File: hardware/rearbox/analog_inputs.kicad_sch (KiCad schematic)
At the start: 4 parts

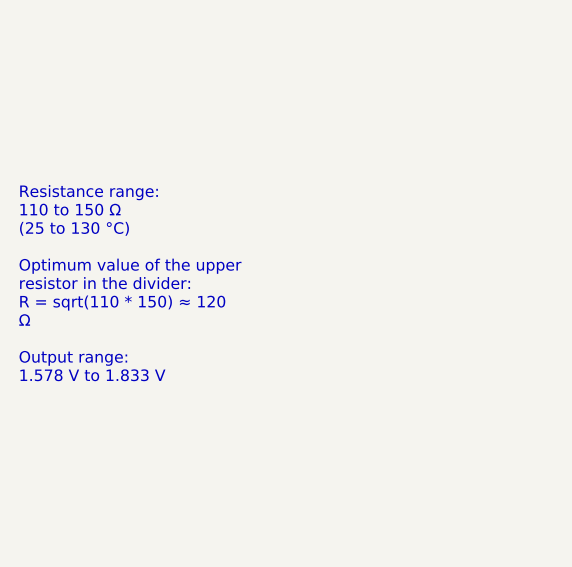
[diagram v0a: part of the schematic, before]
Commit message: Changed power section
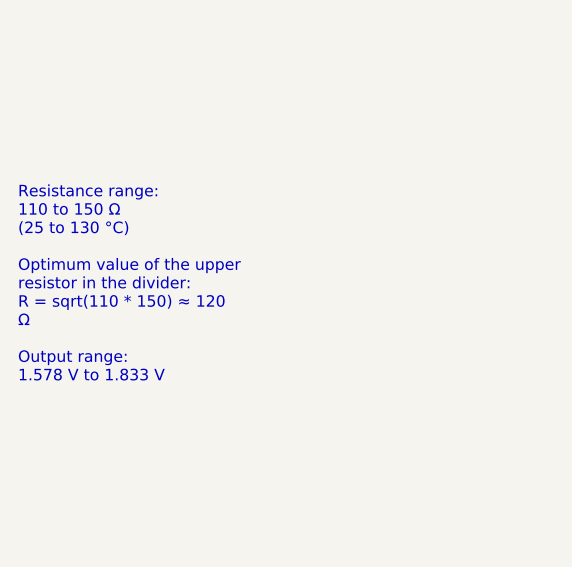
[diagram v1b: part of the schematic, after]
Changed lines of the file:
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@@
 (kicad_sch
-	(version 20231120)
+	(version 20250114)
 	(generator "eeschema")
-	(generator_version "8.0")
+	(generator_version "9.0")
 	(paper "A4")
 	(title_block
@@
 		(company "Author: I. Kajdan")
 		(comment 1 "Reviewer:")
+	)
+	(text "PT100"
+		(exclude_from_sim no)
+		(at 170.18 73.66 0)
+		(effects
+			(font
+				(size 1.27 1.27)
+			)
+			(justify right bottom)
+		)
+	)
+	(text "PT100"
+		(exclude_from_sim no)
+		(at 170.18 127 0)
+		(effects
+			(font
+				(size 1.27 1.27)
+			)
+			(justify right bottom)
+		)
+	)
+	(text "G = 2\nR_{F} = 4k7\nR_{G} = 4k7"
+		(exclude_from_sim no)
+		(at 204.47 87.63 0)
+		(effects
+			(font
+				(size 1.27 1.27)
+			)
+			(justify left bottom)
+		)
+	)
+	(text "G = 2\nR_{F} = 4k7\nR_{G} = 4k7"
+		(exclude_from_sim no)
+		(at 204.47 140.97 0)
+		(effects
+			(font
+				(size 1.27 1.27)
+			)
+			(justify left bottom)
+		)
+	)
+	(text_box "Resistance range:\n110 to 150 Ω\n(25 to 130 °C)\n\nOptimum value of the upper resistor in the divider:\nR = sqrt(110 * 150) ≈ 120 Ω\n\nOutput range:\n1.578 V to 1.833 V"
+		(exclude_from_sim no)
+		(at 48.26 99.06 0)
+		(size 31.75 22.86)
+		(margins 0.9524 0.9524 0.9524 0.9524)
+		(stroke
+			(width -0.0001)
+			(type default)
+		)
+		(fill
+			(type none)
+		)
+		(effects
+			(font
+				(size 1.27 1.27)
+			)
+			(justify left top)
+		)
 	)
 	(junction
@@
 			"FqxEIhEKhXw+Hz6Lx+MT2VgOh8PhcDiczwIIbPf5fJFIRK1WC4KQTCZVsF0xxpRKZTAYDAaDE91O"
 			"DofD4XA4nM8earWaSVFZPNCKw+FwOBwOZ4zhAovD4XA4HA5njOECi8PhcDgcDmeM+X+zbrmZJZpn"
-			"oAAAAABJRU5ErkJggg=="
-		)
-	)
-	(text_box "Resistance range:\n110 to 150 Ω\n(25 to 130 °C)\n\nOptimum value of the upper resistor in the divider:\nR = sqrt(110 * 150) ≈ 120 Ω\n\nOutput range:\n1.578 V to 1.833 V"
-		(exclude_from_sim no)
-		(at 48.26 99.06 0)
-		(size 31.75 22.86)
-		(stroke
-			(width -0.0001)
-			(type default)
-		)
-		(fill
-			(type none)
-		)
+			"oAAAAABJRU5ErkJgggB5AGsAZABHAEgAagBFAHQAWABzAC8AMQBRADYAUQBYAHUAQwBTAEoAVQB2"
+			"ADIANwBkAHQASABLAFUAMABrAEUAbgBQAG4AegBwADAAegBaAHcANgBsAEYAQwAxAEgATwBwADMA"
+			"RwBtAFkATwBtAEkAaAA2AFAAKwA2AHUANQBZAEIATQBTAGkAVQBSAFgAVgB4AGMAVwB6AHMARgB6"
+			"AHgAZgBpAGsAMABkAEoAYgBsAGkAVwBQAHYAOABHAEEASAB0AEQARAB2AGoAVgBOAEUAegAwAC8A"
+			"bgBQAGwAWQBTAGsAUAA0AGEAbAA3AEwASAB3AFoASwBUAHIAbQBDAGwAKwBWAGUANQBTAHQAbwBQ"
+			"AEgAQQBzAG8AWgA0AEMAZwBKAGEAVwBGAGsAMwBUAEUAbwBsAEUASwBCAFIAeQBIAEMAZQBUAHkA"
+			"ZQBCAGkARQBaAFAATgAwAFgASABCAFQAOAA1AFoAaQAzAEMANwBXAGQATwAwADkAdgBiADIAKwAr"
+			"ACsALwAzADcASwBzADIAMgArAC8AMwBYADgATQBWAGcAaQBSAFMAcQBWAFEAVABqAFEAcQBpAFUA"
+			"UQBDAGoAUwBWAGEAUgB3AEQAQQBrADAAbwBZAHgARQBhAGoAdwBuAE4AeQAxAFkAegBVAHkANAA3"
+			"AGoALwBPAGQALwAvAGkAZQBHAEUAOQA1ADcANwA3ADMANwA3ADcAKwAvAHAAYQBYAGwAYQAxAC8A"
+			"NwBHAHEANABpAG8AdABGAG8ASwBCAFQAQwB1AFUAQQBwAFAAWAByADAASwBNADYAVQBhAEQAUwBL"
+			"AEUAMQBrACsAeABGAGcAcwBoAHMAOABsAE4AMQBkAGQAeQBRAEcAOABZAGMATwBHAFAALwAvADUA"
+			"egA5AC8AKwA5AHIAZQBMAGkANAB2AFIAKwBLAEcASAB4ADMAMQBsADEAYwBMAGgATQBQAGEAcQBw"
+			"AG0AbQBIAEQAeAAvAEcANgBqAGgAeQArAHcAWgA3ADMAbgBYAGQAegBzADUATwBUAE8ARABJAHcA"
+			"VQBGAFUAcQBRAEIAeAB3AE0AeQBmAFAAMwAvACsALwBQAGsAbwBlAFUAdABMAHkANgBKAEYAaQA3"
+			"AFoAdAAyADcAWgByADEANgA0AHgAWQA4AGEAawAwADIAbABaAHoAUQBnAEoAQgBBAEoAeQBKADEA"
+			"bwBlAFUAawBOAEYAaABNAEcAVgAzAEIAdwB5AGsASQA4AEEAbABZAHoAcgB1AGkATgBIAGoAdgB6"
+			"AFcAdAA3ADYARgBSAFIAYQBhAG0ANQB1AC8ALwBlADEAdgBiADkAbQB5ADUAYwBZAGIAYgA4AFQA"
+			"cABpAFIATQBCAGQAdw=="
+		)
+	)
+	(hierarchical_label "OFFSET2"
+		(shape input)
+		(at 196.85 125.73 180)
 		(effects
 			(font
 				(size 1.27 1.27)
 			)
-			(justify left top)
-		)
-	)
-	(text "PT100"
-		(exclude_from_sim no)
-		(at 170.18 73.66 0)
+			(justify right)
+		)
+	)
+	(hierarchical_label "OFFSET1"
+		(shape input)
+		(at 196.85 72.39 180)
 		(effects
 			(font
 				(size 1.27 1.27)
 			)
-			(justify right bottom)
-		)
-	)
-	(text "PT100"
-		(exclude_from_sim no)
-		(at 170.18 127 0)
+			(justify right)
+		)
+	)
+	(hierarchical_label "IN2"
+		(shape input)
+		(at 168.91 119.38 180)
 		(effects
 			(font
 				(size 1.27 1.27)
 			)
-			(justify right bottom)
-		)
-	)
-	(text "G = 2\nR_{F} = 4k7\nR_{G} = 4k7"
-		(exclude_from_sim no)
-		(at 204.47 87.63 0)
+			(justify right)
+		)
+	)
+	(hierarchical_label "OUT2"
+		(shape output)
+		(at 223.52 119.38 0)
 		(effects
 			(font
 				(size 1.27 1.27)
 			)
-			(justify left bottom)
-		)
-	)
-	(text "G = 2\nR_{F} = 4k7\nR_{G} = 4k7"
-		(exclude_from_sim no)
-		(at 204.47 140.97 0)
+			(justify left)
+		)
+	)
+	(hierarchical_label "IN1"
+		(shape input)
+		(at 168.91 66.04 180)
 		(effects
 			(font
 				(size 1.27 1.27)
 			)
-			(justify left bottom)
-		)
-	)
-	(hierarchical_label "OFFSET2"
-		(shape input)
-		(at 196.85 125.73 180)
-		(fields_autoplaced yes)
-		(effects
-			(font
-				(size 1.27 1.27)
-			)
-			(justify right)
-		)
-	)
-	(hierarchical_label "OFFSET1"
-		(shape input)
-		(at 196.85 72.39 180)
-		(fields_autoplaced yes)
-		(effects
-			(font
-				(size 1.27 1.27)
-			)
-			(justify right)
-		)
-	)
-	(hierarchical_label "IN2"
-		(shape input)
-		(at 168.91 119.38 180)
-		(fields_autoplaced yes)
-		(effects
-			(font
-				(size 1.27 1.27)
-			)
-			(justify right)
-		)
-	)
-	(hierarchical_label "OUT2"
-		(shape output)
-		(at 223.52 119.38 0)
-		(fields_autoplaced yes)
-		(effects
-			(font
-				(size 1.27 1.27)
-			)
-			(justify left)
-		)
-	)
-	(hierarchical_label "IN1"
-		(shape input)
-		(at 168.91 66.04 180)
-		(fields_autoplaced yes)
-		(effects
-			(font
-				(size 1.27 1.27)
-			)
 			(justify right)
 		)
@@
 		(shape output)
 		(at 223.52 66.04 0)
-		(fields_autoplaced yes)
 		(effects
 			(font
@@
 		(at 198.12 62.23)
 		(size 24.13 13.97)
+		(exclude_from_sim no)
+		(in_bom yes)
+		(on_board yes)
+		(dnp no)
 		(stroke
 			(width 0.1524)
@@
 		(at 198.12 115.57)
 		(size 24.13 13.97)
+		(exclude_from_sim no)
+		(in_bom yes)
+		(on_board yes)
+		(dnp no)
 		(stroke
 			(width 0.1524)
